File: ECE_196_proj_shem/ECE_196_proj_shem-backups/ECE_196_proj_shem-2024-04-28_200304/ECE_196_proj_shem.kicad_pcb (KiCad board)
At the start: 2 copper layers, 44.2 x 55.1 mm, 13 parts, among them J2 Screw_Terminal_01x06, U1 MAX9814

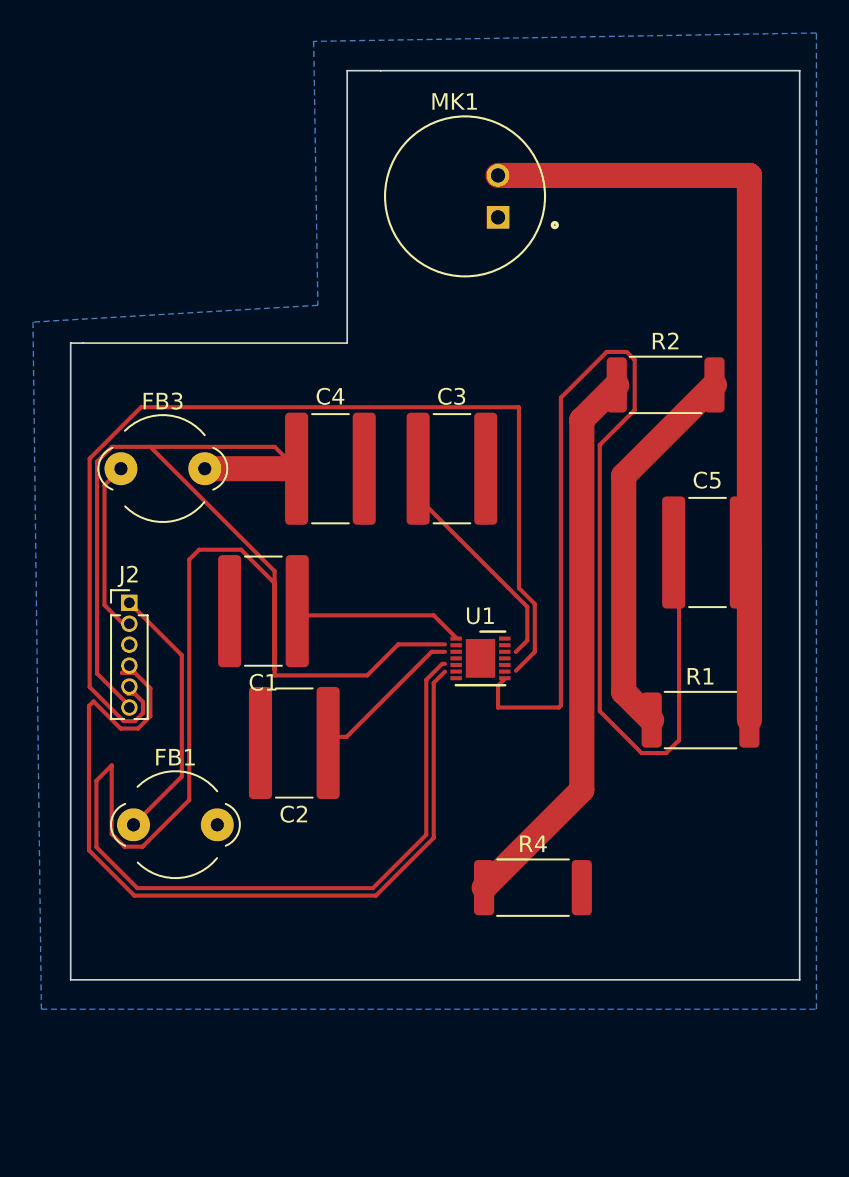
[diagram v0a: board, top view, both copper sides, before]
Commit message: Adding these files for backup.
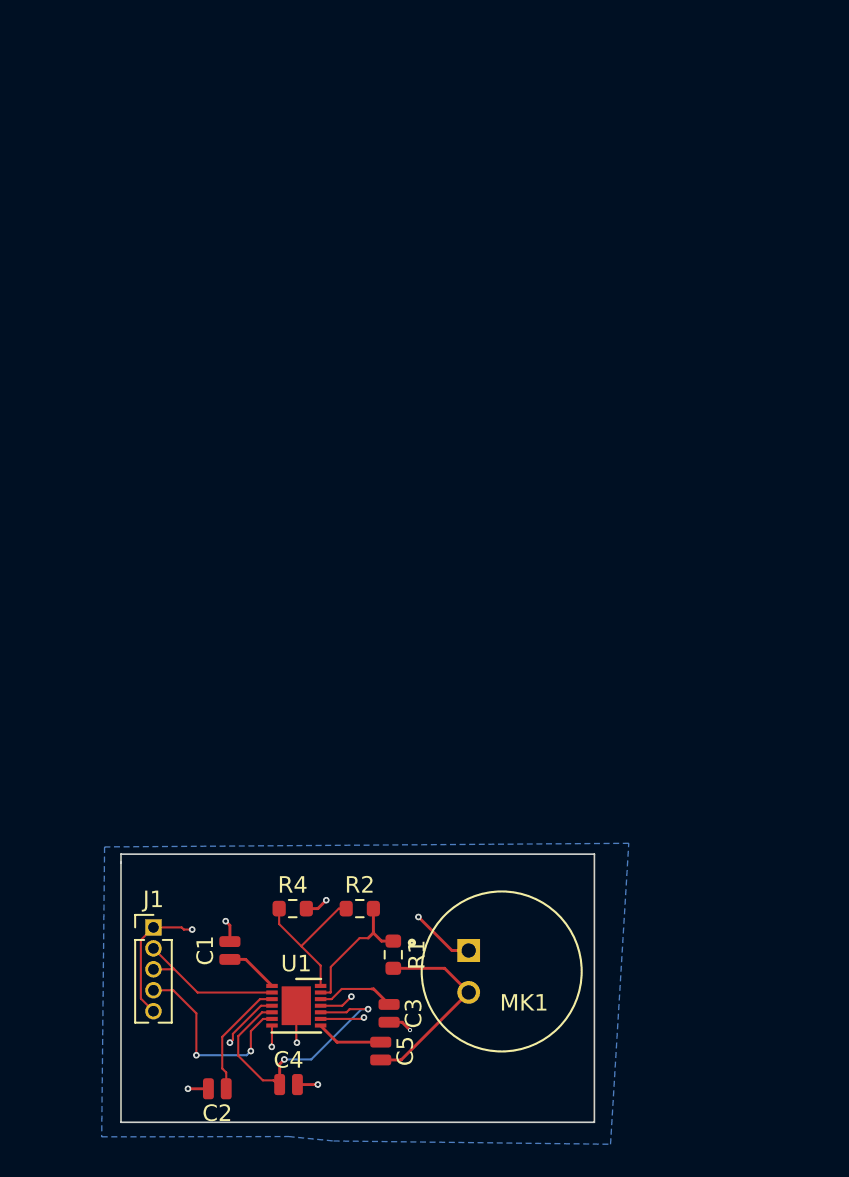
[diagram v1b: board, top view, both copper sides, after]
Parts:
- removed FB1, FB3: FerriteBead, Ferrite_THT:LairdTech_28C0236-0JW-10
- removed J2: Screw_Terminal_01x06, Connector_PinHeader_1.27mm:PinHeader_1x06_P1.27mm_Vertical
- added J1: Screw_Terminal_01x05, Connector_PinHeader_1.27mm:PinHeader_1x05_P1.27mm_Vertical, F.Cu at (144.2, 86.2)
- C1: value 0.1uF -> 470nF; footprint Capacitor_SMD:C_1825_4564Metric -> Capacitor_SMD:C_0504_1310Metric
- C2: value 22uF -> 2.2uF; footprint Capacitor_SMD:C_1825_4564Metric -> Capacitor_SMD:C_0504_1310Metric
- C3, C5: footprint Capacitor_SMD:C_1825_4564Metric -> Capacitor_SMD:C_0504_1310Metric
- C4: value 2.2uF -> 1uF; footprint Capacitor_SMD:C_1825_4564Metric -> Capacitor_SMD:C_0504_1310Metric
- R1: value 22k -> 2.2k; footprint Resistor_SMD:R_2512_6332Metric -> Resistor_SMD:R_0603_1608Metric
- R2, R4: footprint Resistor_SMD:R_2512_6332Metric -> Resistor_SMD:R_0603_1608Metric
- moved MK1 47.0 mm to (165.3, 88.9), turned to 180 degrees
- moved C4 37.4 mm to (152.4, 95.8)
- moved R2 36.8 mm to (156.7, 85.1)
- moved C5 36.1 mm to (158.0, 93.7), turned to -90 degrees
- moved C3 33.2 mm to (158.5, 91.4), turned to -90 degrees
- moved U1 23.8 mm to (152.9, 91.0)
- moved R1 23.4 mm to (158.8, 87.9), turned to -90 degrees
- moved C2 21.5 mm to (148.1, 96.0)
- moved C1 20.7 mm to (148.8, 87.6), turned to 90 degrees
- moved R4 14.6 mm to (152.7, 85.1)
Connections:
- C4 pad 1: /VDD -> /GAIN
- U1 pad 2: /VDD -> /GAIN
- U1 pad 5: /VDD -> /GAIN
- U1 pad 9: /A/R -> GND
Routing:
- net /VDD: track 137.1 -> 0.00 mm
- net Net-(U1-MICIN): track 70.3 -> 4.05 mm
- net /A/R: track 65.0 -> 0.00 mm
- net /OUTPUT: track 51.8 -> 11.9 mm, vias 0 -> 2
- net Net-(C5-Pad2): track 48.3 -> 12.2 mm
- net GND: track 0.00 -> 31.0 mm, vias 0 -> 12
- net /GAIN: track 0.00 -> 27.2 mm, vias 0 -> 2
- net Net-(U1-TH): track 33.8 -> 9.40 mm
- net Net-(J2-Pin_1): track 16.0 -> 0.00 mm
- net Net-(U1-MICBIAS): track 23.3 -> 8.48 mm
- net Net-(J2-Pin_2): track 10.7 -> 0.00 mm
- net Net-(U1-BIAS): track 14.1 -> 4.80 mm
- net Net-(U1-CT): track 10.3 -> 3.21 mm
- net Net-(U1-CG): track 9.06 -> 7.21 mm
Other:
- board size 44.2 x 55.1 mm -> 28.7 x 16.3 mm
